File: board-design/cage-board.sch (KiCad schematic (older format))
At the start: 54 parts, among them J1 Jack-DC, J10 73131-0240, J11 73131-0240, J12 73131-0240, J13 Conn_01x02, J14 Conn_01x02, J15 Conn_02x13_test_points, J2 Conn_02x17_Ribbon, J3 TB002-500-03BE, J4 73131-0240, J5 73131-0240, J6 73131-0240, J7 TB002-500-03BE, J8 73131-0240, J9 TB002-500-03BE, Q1 BD139, Q2 BD139, Q3 2N3906, Q4 2N3906, U1 74HC04, U2 VX7805-500, U3 4N25, U4 4N25

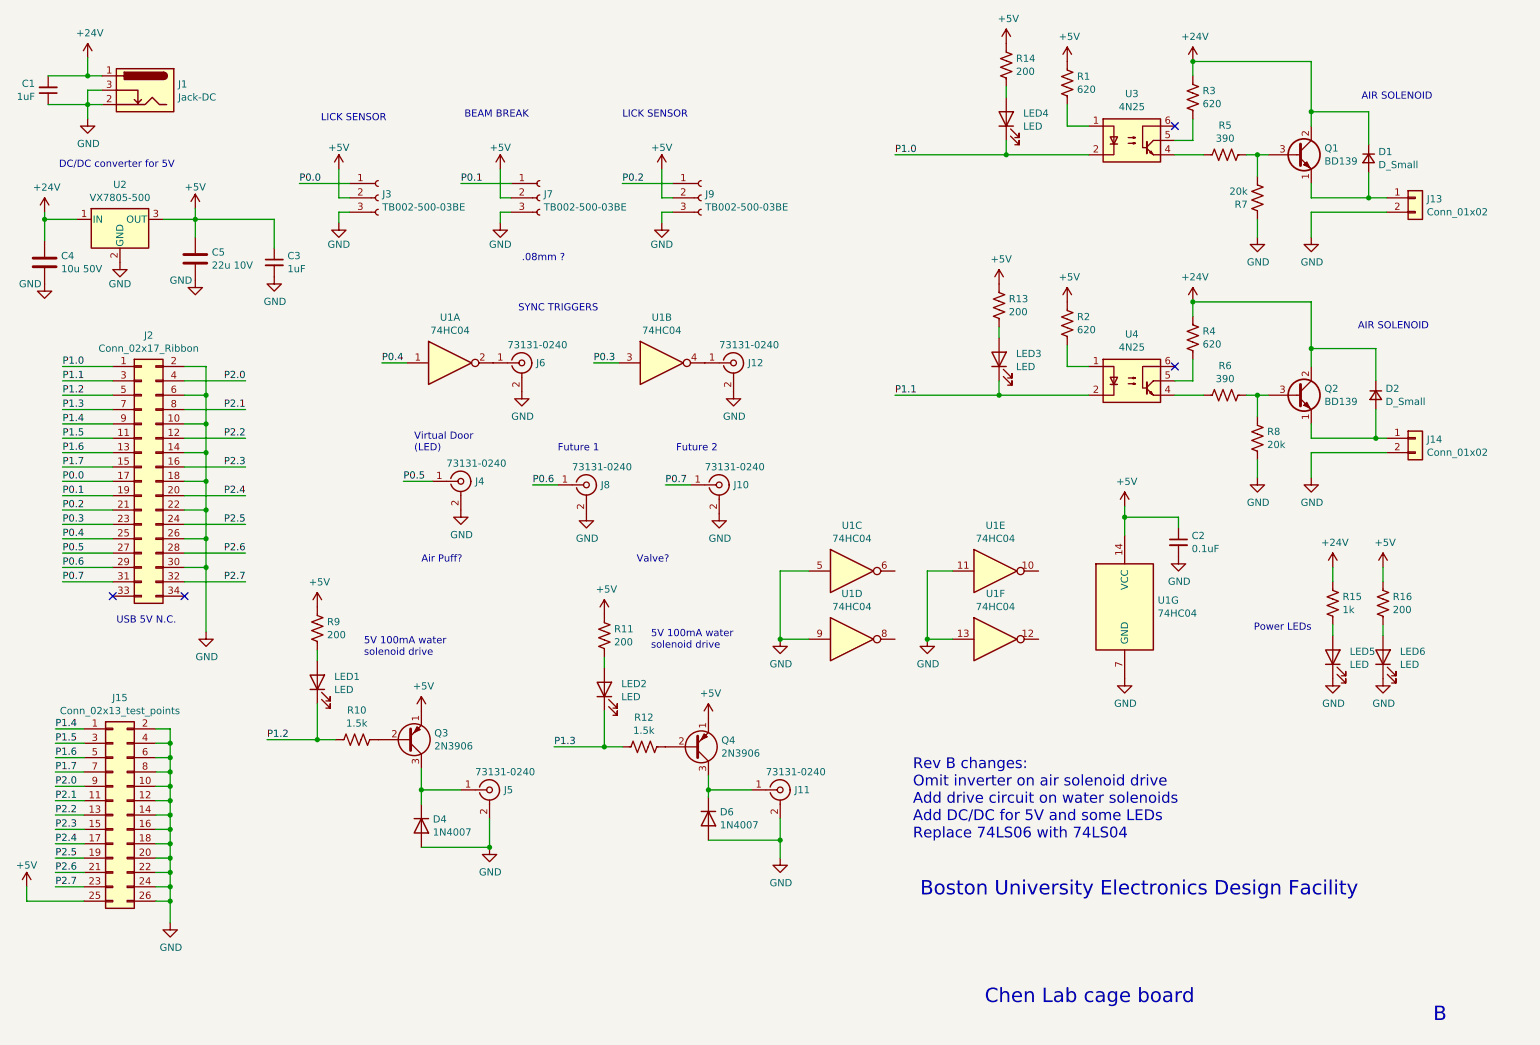
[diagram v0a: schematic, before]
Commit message: auto push run at Fri Apr  9 11:10:50 EDT 2021
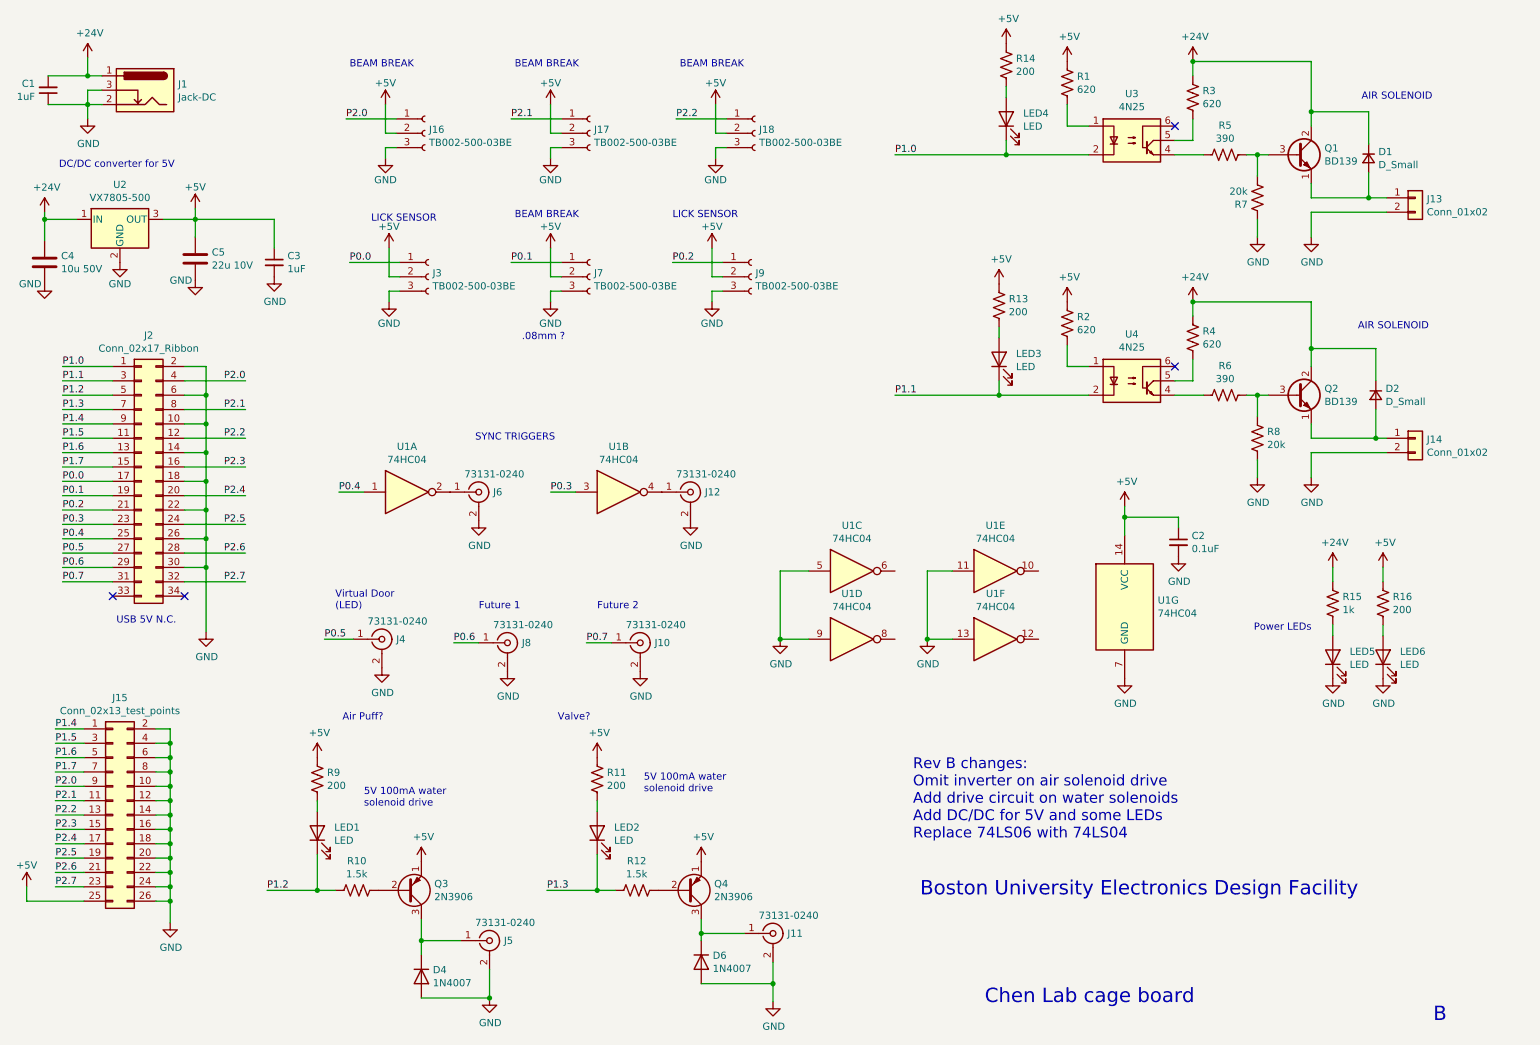
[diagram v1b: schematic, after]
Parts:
- added J16, J17, J18: TB002-500-03BE, TerminalBlock:TerminalBlock_bornier-3_P5.08mm, symbol Connector:Conn_01x03_Female
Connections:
- net +5V: now also J16.2 (Pin_2), J17.2 (Pin_2), J18.2 (Pin_2)
- net GND: now also J16.3 (Pin_3), J17.3 (Pin_3), J18.3 (Pin_3)
- net P2.0: now also J16.1 (Pin_1)
- net P2.1: now also J17.1 (Pin_1)
- net P2.2: now also J18.1 (Pin_1)
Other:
- moved on the sheet: D4, D6, J10, J11, J12, J3, J4, J5, J6, J7, J8, J9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
